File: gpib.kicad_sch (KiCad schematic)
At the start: 5 parts, among them U1 SN74LVC8T245PWR, U2 SN74LVC07APWR, U6 SN74LVC1G07DCKR, U7 SN74LVC14APWR

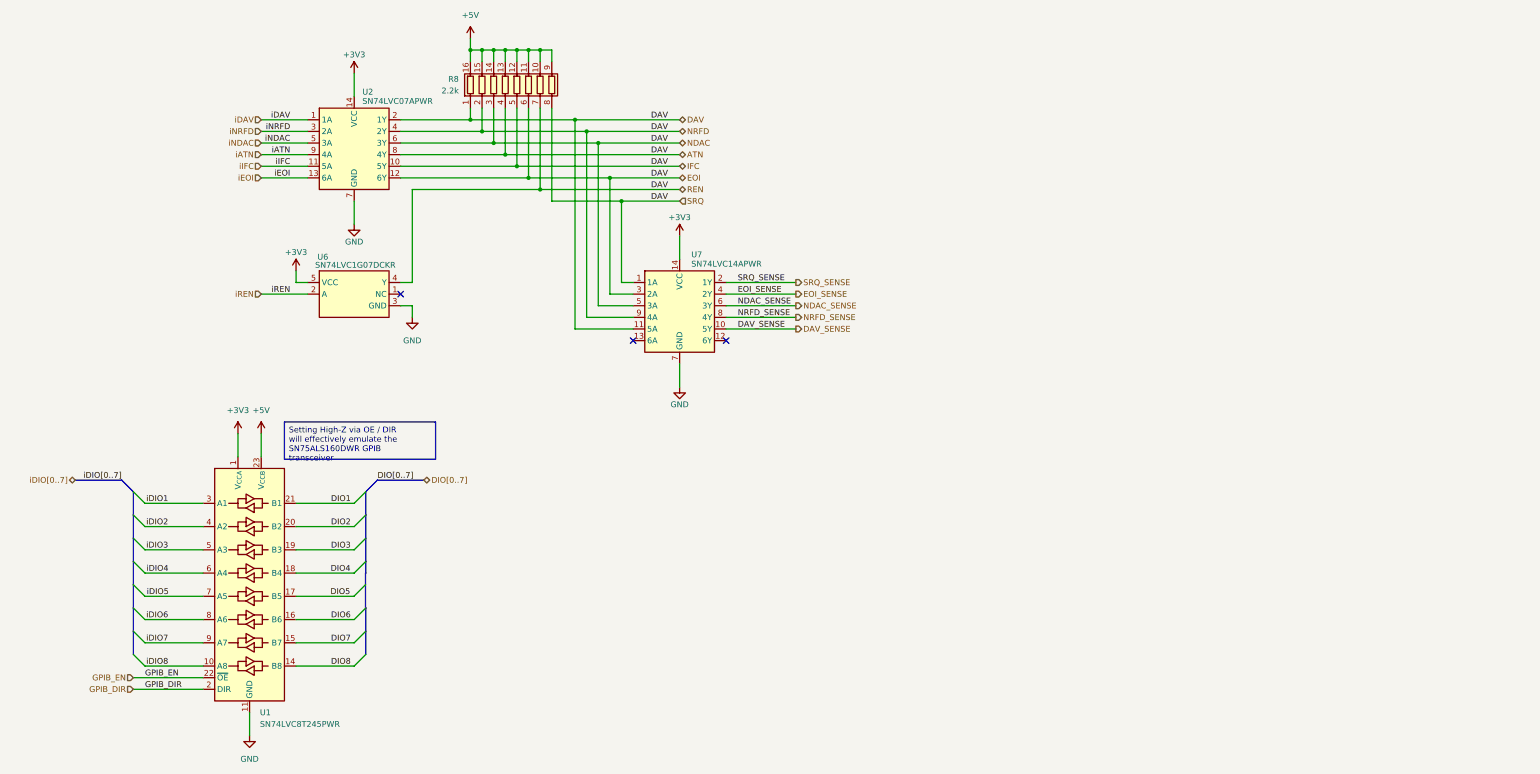
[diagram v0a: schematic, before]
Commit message: Start work on PCB
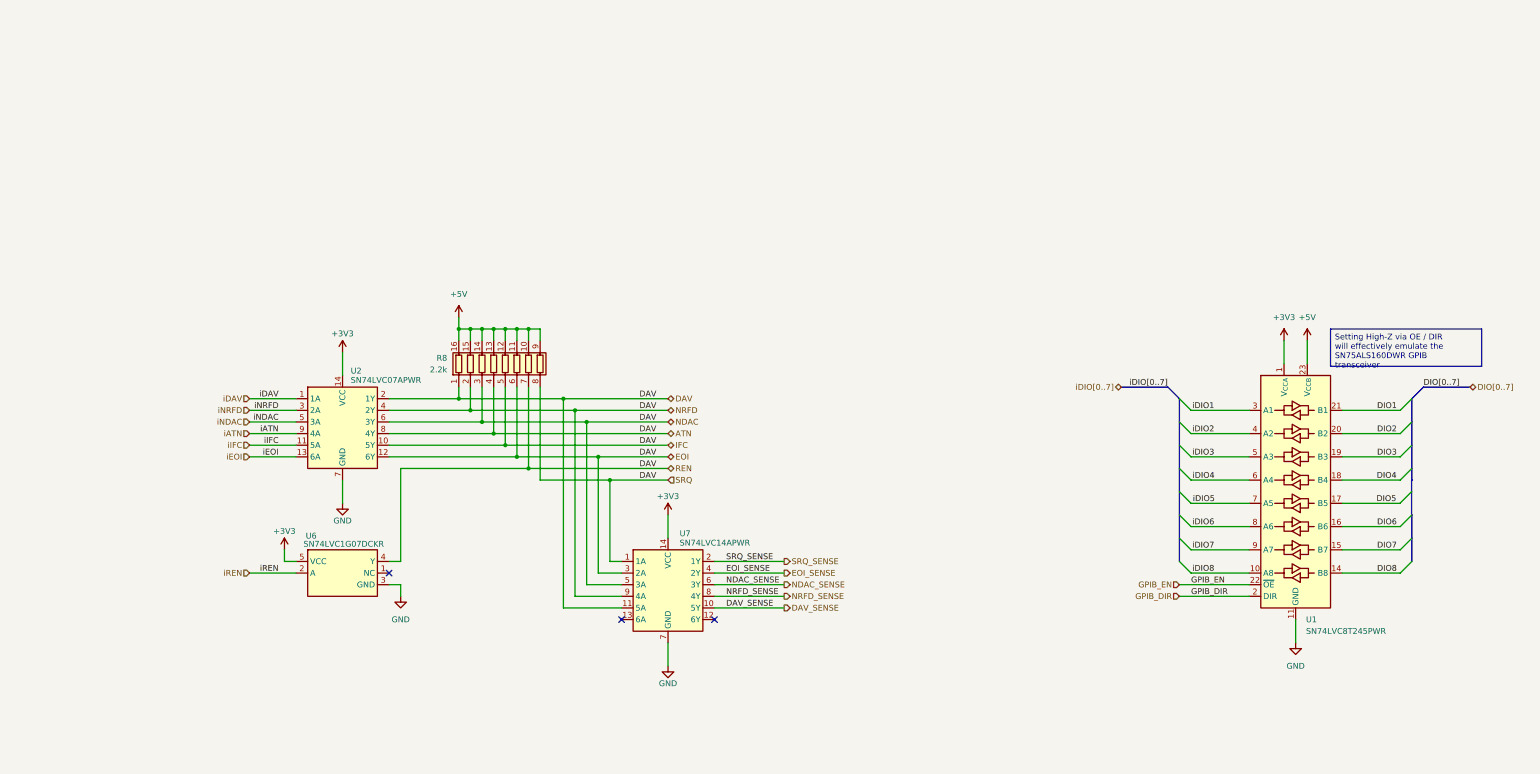
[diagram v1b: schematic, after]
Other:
- moved on the sheet: R8, U1, U2, U6, U7
